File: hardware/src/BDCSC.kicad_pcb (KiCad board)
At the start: 2 copper layers, 64 x 46 mm, 47 parts, among them J1 Conn_02x03_Odd_Even, J10 Conn_02x01, J11 Conn_02x01, J12 Conn_02x04_Odd_Even, J2 Conn_02x03_Odd_Even, J3 Conn_01x05, J4 Conn_02x01, J5 Conn_02x01, J6 Conn_01x06_Pin, J7 Conn_02x01, J8 Conn_01x03, J9 Conn_02x01, U1 INA180A1, U2 LM358, U3 DRV8870DDA, U4 PY32F003F1xPx

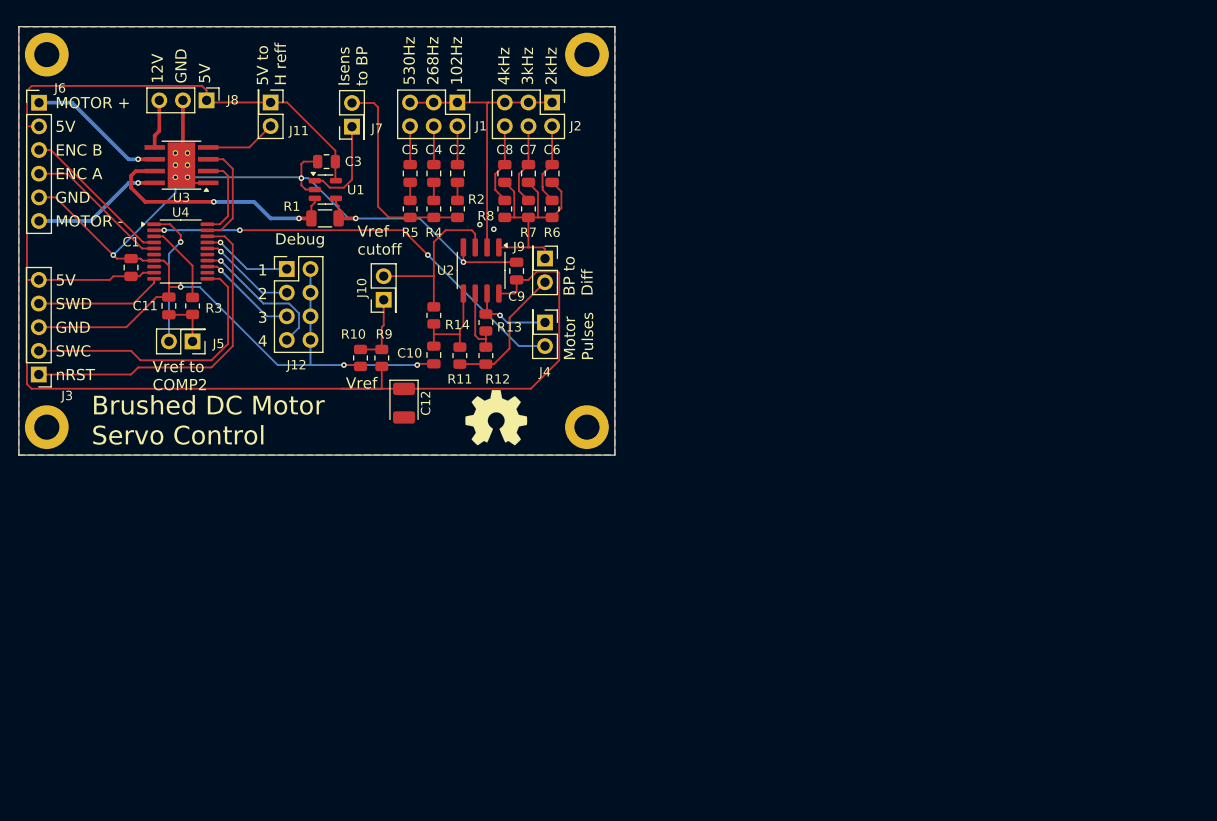
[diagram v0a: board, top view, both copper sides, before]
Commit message: Updated dev board and cad model
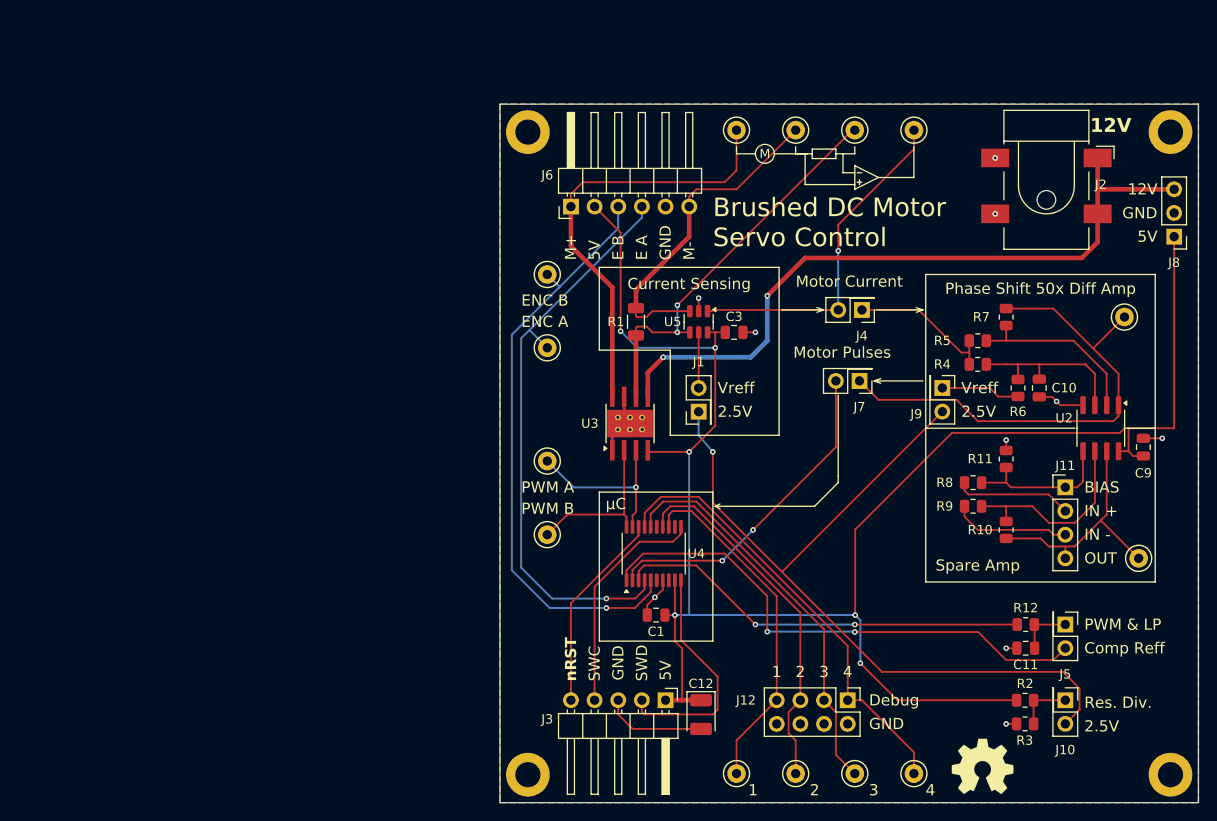
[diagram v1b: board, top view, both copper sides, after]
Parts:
- removed C2: 470nF, Capacitor_SMD:C_0805_2012Metric
- removed C4: 180nF, Capacitor_SMD:C_0805_2012Metric
- removed C5: 91nF, Capacitor_SMD:C_0805_2012Metric
- removed C6: 24nF, Capacitor_SMD:C_0805_2012Metric
- removed C7: 16nF, Capacitor_SMD:C_0805_2012Metric
- removed C8: 12nF, Capacitor_SMD:C_0805_2012Metric
- removed R13, R14: 1M, Resistor_SMD:R_0805_2012Metric
- removed U1: INA180A1, Package_TO_SOT_SMD:SOT-23-5
- added TP1: TestPoint, TestPoint:TestPoint_Keystone_5000-5004_Miniature, F.Cu at (98.2, 112.3)
- added TP10: TestPoint, TestPoint:TestPoint_Keystone_5000-5004_Miniature, F.Cu at (117.3, 181.4)
- added TP11: TestPoint, TestPoint:TestPoint_Keystone_5000-5004_Miniature, F.Cu at (110.9, 181.4)
- added TP12: TestPoint, TestPoint:TestPoint_Keystone_5000-5004_Miniature, F.Cu at (104.6, 181.4)
- added TP13: TestPoint, TestPoint:TestPoint_Keystone_5000-5004_Miniature, F.Cu at (98.2, 181.4)
- added TP14: TestPoint, TestPoint:TestPoint_Keystone_5000-5004_Miniature, F.Cu at (141.4, 158.3)
- added TP2: TestPoint, TestPoint:TestPoint_Keystone_5000-5004_Miniature, F.Cu at (104.6, 112.3)
- added TP3: TestPoint, TestPoint:TestPoint_Keystone_5000-5004_Miniature, F.Cu at (110.9, 112.3)
- added TP4: TestPoint, TestPoint:TestPoint_Keystone_5000-5004_Miniature, F.Cu at (117.3, 112.3)
- added TP5: TestPoint, TestPoint:TestPoint_Keystone_5000-5004_Miniature, F.Cu at (77.9, 135.7)
- added TP6: TestPoint, TestPoint:TestPoint_Keystone_5000-5004_Miniature, F.Cu at (77.9, 127.8)
- added TP7: TestPoint, TestPoint:TestPoint_Keystone_5000-5004_Miniature, F.Cu at (77.9, 147.8)
- added TP8: TestPoint, TestPoint:TestPoint_Keystone_5000-5004_Miniature, F.Cu at (77.9, 155.7)
- added TP9: TestPoint, TestPoint:TestPoint_Keystone_5000-5004_Miniature, F.Cu at (139.9, 132.4)
- added U5: INA181, Package_TO_SOT_SMD:SOT-23-6, F.Cu at (94.1, 132.9)
- J1: value Conn_02x03_Odd_Even -> Conn_02x01; footprint Connector_PinHeader_2.54mm:PinHeader_2x03_P2.54mm_Vertical -> Connector_PinHeader_2.54mm:PinHeader_2x01_P2.54mm_Vertical
- J11: value Conn_02x01 -> Conn_01x04_Pin; footprint Connector_PinHeader_2.54mm:PinHeader_2x01_P2.54mm_Vertical -> Connector_PinHeader_2.54mm:PinHeader_1x04_P2.54mm_Vertical
- J2: value Conn_02x03_Odd_Even -> Barrel_Jack_Switch; footprint Connector_PinHeader_2.54mm:PinHeader_2x03_P2.54mm_Vertical -> Connector_BarrelJack:BarrelJack_CLIFF_FC681465S_SMT_Horizontal
- J3: footprint Connector_PinHeader_2.54mm:PinHeader_1x05_P2.54mm_Vertical -> Connector_PinHeader_2.54mm:PinHeader_1x05_P2.54mm_Horizontal
- J6: footprint Connector_PinHeader_2.54mm:PinHeader_1x06_P2.54mm_Vertical -> Connector_PinHeader_2.54mm:PinHeader_1x06_P2.54mm_Horizontal
- R1: value .680R -> 0.15R
- R12: value 20K -> 3K3
- R2, R3, R4, R5, R8: value 3K3 -> 20K
- R6, R7: value 3K3 -> 1M
- moved J8 104.9 mm to (145.2, 123.7), turned to 180 degrees
- moved R3 100.0 mm to (129.2, 176.0), turned to 0 degrees
- moved C11 99.1 mm to (129.3, 167.9), turned to 0 degrees
- moved J5 98.5 mm to (133.5, 165.4), turned to -90 degrees
- moved J11 94.8 mm to (133.5, 150.6), turned to 0 degrees
- moved J10 84.9 mm to (133.5, 173.5), turned to -90 degrees
- moved R2 80.6 mm to (129.2, 173.5), turned to 180 degrees
- moved J12 76.0 mm to (110.1, 173.5), turned to -90 degrees
- moved J3 75.8 mm to (90.6, 173.5), turned to -90 degrees
- moved REF** 72.9 mm to (144.8, 181.5)
- moved R10 71.7 mm to (127.2, 155.2)
- moved C9 69.9 mm to (141.9, 146.3)
- moved U2 68.7 mm to (137.3, 144.3)
- moved C1 67.6 mm to (89.6, 164.4), turned to 180 degrees
- moved R9 65.5 mm to (123.6, 152.7), turned to 180 degrees
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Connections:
- C10 pad 1: Net-(U2B-+) -> Net-(U2A-+)
- J1 pad 1: Net-(J1-Pin_1) -> +2V5
- J10 pad 2: Net-(J10-Pin_2) -> +2V5
- J11 pad 1: +5V -> Net-(J11-Pin_1)
- J2 pad 1: Net-(J1-Pin_1) -> +12V
- J2 pad 2: Net-(J2-Pin_2) -> GND
- J2 pad 3: Net-(J1-Pin_1) -> GND
- J3 pad 1: /~{RST} -> +5V
- J3 pad 2: /SWC -> /SWD
- J3 pad 4: /SWD -> /SWC
- J3 pad 5: +5V -> /~{RST}
- J4 pad 1: /MOTOR_PULSES -> /Diff Amp In
- J4 pad 2: /MOTOR_PULSE_COMP -> /Motor Current
- J6 pad 1: /MOTOR_P -> /Motor +
- J6 pad 6: /MOTOR_N -> /Motor -
- J7 pad 1: Net-(J7-Pin_1) -> /Diff Amp Out
- J7 pad 2: /bpf_in -> /Motor Pulses µC
- J9 pad 1: /bpf_out -> /Diff Amp Vreff
- J9 pad 2: Net-(J9-Pin_2) -> +2V5
- R1 pad 1: Net-(U1-+) -> Net-(U3-OUT1)
- R1 pad 2: GND -> /Motor -
- R10 pad 1: GND -> Net-(J11-Pin_4)
- R10 pad 2: Net-(J10-Pin_1) -> Net-(U2B--)
- R11 pad 1: Net-(U2B-+) -> GND
- R11 pad 2: Net-(J9-Pin_2) -> Net-(J11-Pin_1)
- R12 pad 1: Net-(U2B--) -> Net-(J5-Pin_1)
- R12 pad 2: Net-(J9-Pin_2) -> Net-(U4-PA4)
- R2 pad 1: /bpf_in -> Net-(J10-Pin_1)
- R2 pad 2: Net-(C2-Pad1) -> +5V
- R3 pad 1: Net-(J5-Pin_1) -> GND
- R3 pad 2: Net-(U4-PA4) -> Net-(J10-Pin_1)
- R4 pad 1: /bpf_in -> Net-(U2A-+)
- R4 pad 2: Net-(C4-Pad1) -> /Diff Amp In
- R5 pad 1: /bpf_in -> Net-(U2A--)
- R5 pad 2: Net-(C5-Pad1) -> /Diff Amp In
- R6 pad 1: /bpf_out -> Net-(U2A-+)
- R6 pad 2: Net-(J2-Pin_2) -> /Diff Amp Vreff
- R7 pad 1: /bpf_out -> Net-(U2A--)
- R7 pad 2: Net-(J2-Pin_4) -> /Diff Amp Out
- R8 pad 1: /bpf_out -> Net-(J11-Pin_1)
- R8 pad 2: Net-(J2-Pin_6) -> Net-(J11-Pin_2)
- R9 pad 1: Net-(J10-Pin_1) -> Net-(U2B--)
- R9 pad 2: +5V -> Net-(J11-Pin_3)
- U2 pad 1: /bpf_out -> /Diff Amp Out
- U2 pad 2: Net-(J1-Pin_1) -> Net-(U2A--)
- U2 pad 3: Net-(J10-Pin_2) -> Net-(U2A-+)
- U2 pad 5: Net-(U2B-+) -> Net-(J11-Pin_1)
- U2 pad 7: /MOTOR_PULSES -> Net-(J11-Pin_4)
- U3 pad 4: Net-(J11-Pin_2) -> +5V
- U3 pad 6: /MOTOR_P -> Net-(U3-OUT1)
- U3 pad 7: Net-(U1-+) -> GND
- U3 pad 8: /MOTOR_N -> /Motor +
- U4 pad 13: /Debug Pin 3 -> /Debug Pin 4
- U4 pad 14: /Debug Pin 4 -> /Debug Pin 3
- U4 pad 2: /MOTOR_PULSE_COMP -> /Motor Pulses µC
- U4 pad 4: /ENC_IN_B -> /ENC_IN_A
- U4 pad 5: /ENC_IN_A -> /ENC_IN_B
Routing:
- net GND: track 151.0 -> 34.3 mm, vias 9 -> 10
- net +2V5: track 0.00 -> 86.7 mm, vias 0 -> 1
- net +12V: track 5.26 -> 76.8 mm, vias 0 -> 2
- net /Diff Amp Out: track 0.00 -> 54.1 mm
- net /ENC_IN_B: track 16.5 -> 64.4 mm, vias 0 -> 1
- net /ENC_IN_A: track 15.7 -> 62.8 mm, vias 0 -> 1
- net /MOTOR_PULSE_COMP: track 47.1 -> 0.00 mm, vias 3 -> 0
- net /Motor +: track 0.00 -> 46.8 mm
- net Net-(U3-OUT1): track 0.00 -> 43.4 mm, vias 0 -> 2
- net Net-(J5-Pin_2): track 15.3 -> 56.4 mm, vias 1 -> 2
- net /Debug Pin 1: track 9.71 -> 48.2 mm, vias 1 -> 0
- net /Motor Current: track 0.00 -> 36.8 mm, vias 0 -> 1
- net Net-(U4-PA4): track 8.84 -> 44.5 mm, vias 0 -> 2
- net /Motor -: track 0.00 -> 35.7 mm
- net /Motor Pulses µC: track 0.00 -> 35.5 mm, vias 0 -> 2
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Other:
- board size 64 x 46 mm -> 75 x 75 mm
- board text added: "2.5V"
- board text added: "BIAS"
- board text added: "Comp Reff"
- board text added: "Current Sensing"
- board text added: "E A"
- board text added: "E B"
- board text added: "IN +"
- board text added: "IN -"
- board text added: "M"
- board text added: "M+"
- board text added: "M-"
- board text added: "Motor Current"
- board text added: "OUT"
- board text added: "PWM & LP"
- board text added: "PWM A"
- board text added: "PWM B"
- board text added: "Phase Shift 50x Diff Amp"
- board text added: "Res. Div."
- board text added: "Spare Amp"
- board text added: "Vreff"
- board text added: "µC"
- board text removed: "102Hz"
- board text removed: "268Hz"
- board text removed: "2kHz"
- board text removed: "3kHz"
- board text removed: "4kHz"
- board text removed: "530Hz"
- board text removed: "5V to H reff"
- board text removed: "BP to Diff"
- board text removed: "Isens to BP"
- board text removed: "MOTOR +"
- board text removed: "MOTOR -"
- board text removed: "Vref"
- board text removed: "Vref cutoff"
- board text removed: "Vref to COMP2"
